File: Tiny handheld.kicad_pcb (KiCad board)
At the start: 2 copper layers, 34.3 x 58.4 mm, 43 parts, among them IC1 BQ21040DBVR, J1 VDisplay/prog1, J2 HDisplay/prog, J3 USB_C_Receptacle_USB2.0, U1 ATtiny85-20P, U2 ATtiny85-20S

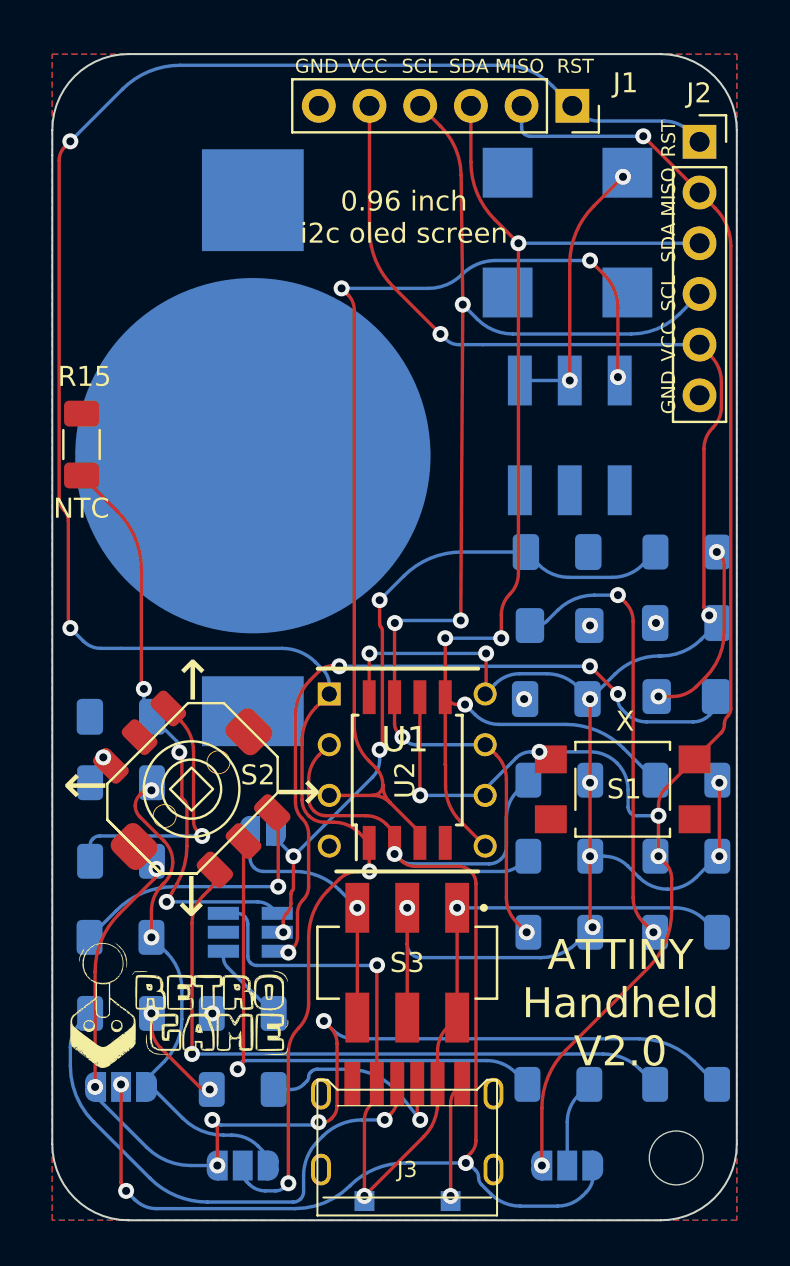
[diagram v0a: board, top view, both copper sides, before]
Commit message: enh tracks
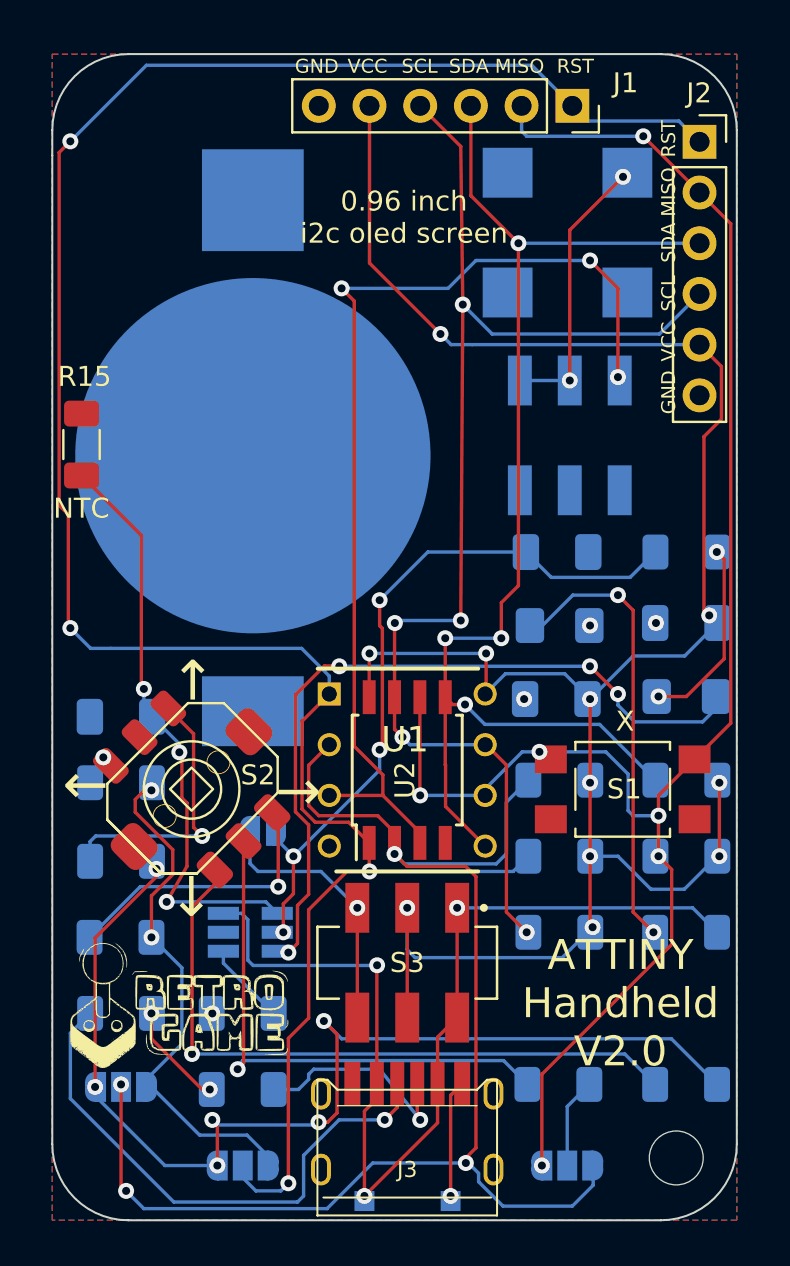
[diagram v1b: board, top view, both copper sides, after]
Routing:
- net PB5/RES: track 114.1 -> 115.8 mm
- net VCC: track 104.0 -> 105.4 mm
- net PB3: track 70.0 -> 71.4 mm
- net PB1/MISO: track 84.5 -> 85.7 mm
- net Net-(JP1-Pad1): track 25.0 -> 26.0 mm
- net PB2/SCL/SCK: track 63.3 -> 64.2 mm
- net Net-(JP1-Pad3): track 54.2 -> 55.1 mm
- net Net-(J3-PadA5): track 26.7 -> 27.5 mm
- net Net-(C6-Pad1): track 35.6 -> 36.3 mm
- net Net-(D2-Pad1): track 37.0 -> 37.6 mm
- net PB4: track 52.1 -> 51.5 mm

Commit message: cleanup
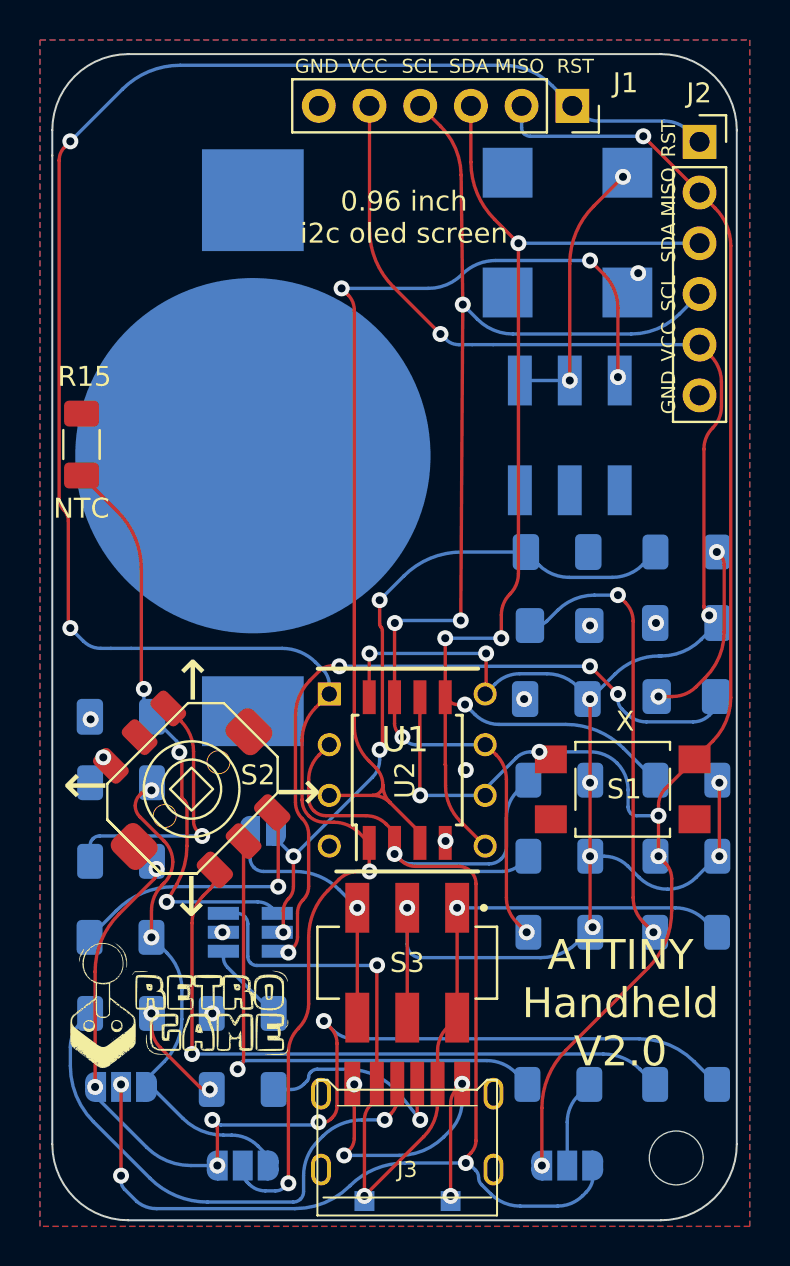
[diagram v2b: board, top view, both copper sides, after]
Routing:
- net GND: track 11.1 -> 22.9 mm, vias 7 -> 15
- net PB5/RES: track 115.8 -> 114.1 mm
- net VCC: track 105.4 -> 104.0 mm
- net PB3: track 71.4 -> 69.9 mm
- net PB1/MISO: track 85.7 -> 84.5 mm
- net Net-(JP1-Pad1): track 26.0 -> 25.0 mm
- net PB2/SCL/SCK: track 64.2 -> 63.3 mm
- net Net-(JP1-Pad3): track 55.1 -> 54.2 mm
- net Net-(J3-PadA5): track 27.5 -> 26.7 mm
- net Net-(C6-Pad1): track 36.3 -> 35.6 mm
- net Net-(D2-Pad1): track 37.6 -> 37.0 mm
- net PB4: track 51.5 -> 52.1 mm
